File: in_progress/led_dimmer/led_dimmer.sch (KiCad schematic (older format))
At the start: 29 parts, among them IC1 ATTINY2313A-P, P1 CONN_3X2, P2 CONN_4, P3 CONN_4, Q1 Q_NPN_CBE, SW1 SPST, X1 CRYSTAL

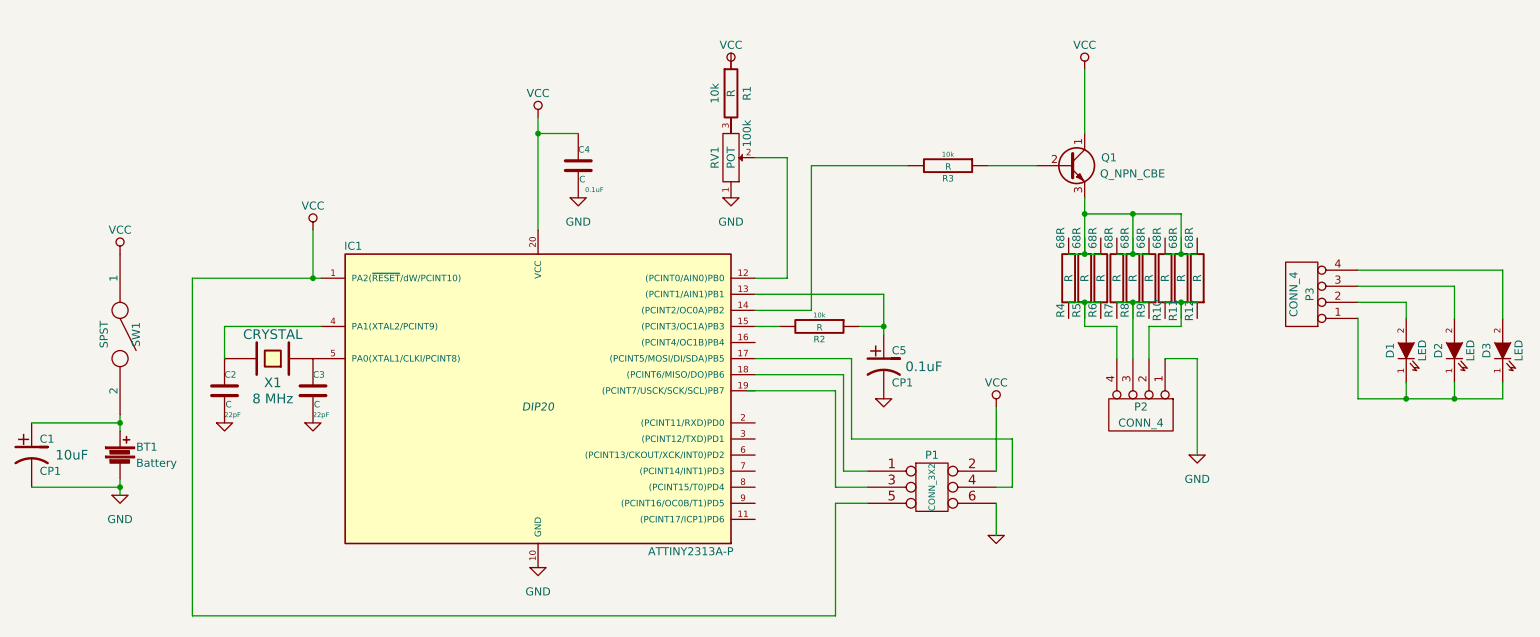
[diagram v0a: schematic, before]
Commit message: .
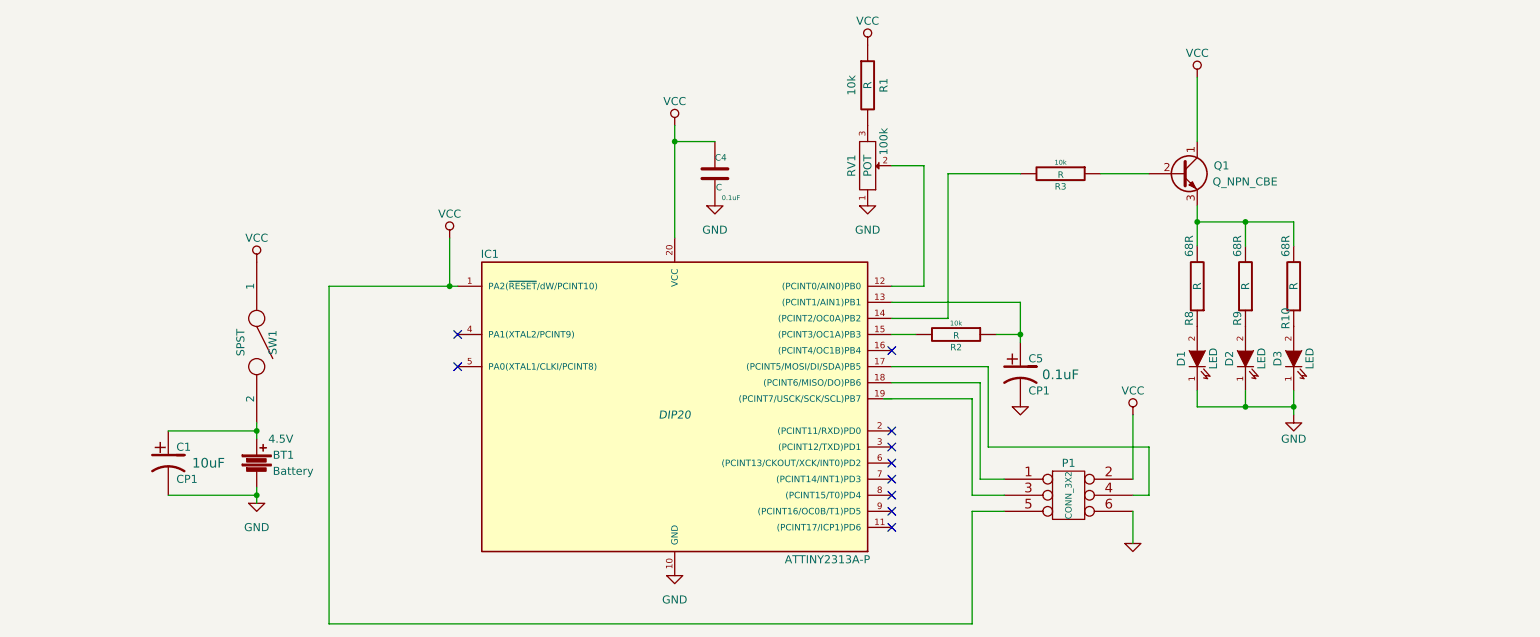
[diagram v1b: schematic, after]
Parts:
- removed C2, C3: C, 22pF, symbol C-RESCUE-led_dimmer
- removed P2, P3: CONN_4, symbol CONN_4
- removed R11, R12, R4, R5, R6, R7: R, 68R, symbol R-RESCUE-led_dimmer
- removed X1: CRYSTAL, 8 MHz, symbol CRYSTAL
- BT1: footprint (none) -> 4.5V
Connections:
- wire segments 70 -> 46
- no-connect marks 0 -> 10
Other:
- moved on the sheet: BT1, C1, C4, C5, D1, D2, D3, IC1, P1, Q1, R1, R10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
